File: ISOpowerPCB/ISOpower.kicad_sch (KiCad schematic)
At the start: 12 parts

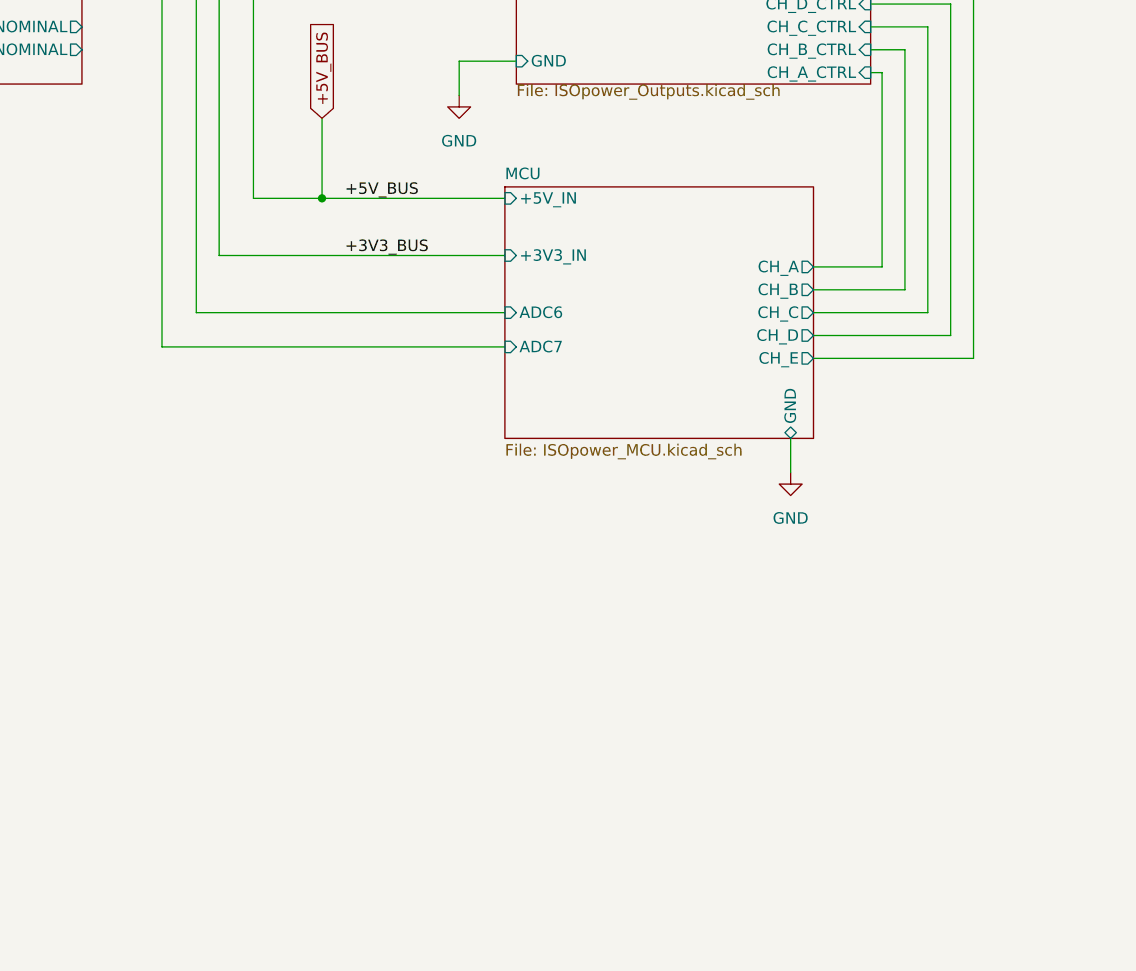
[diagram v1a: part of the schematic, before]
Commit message: modified pcb files
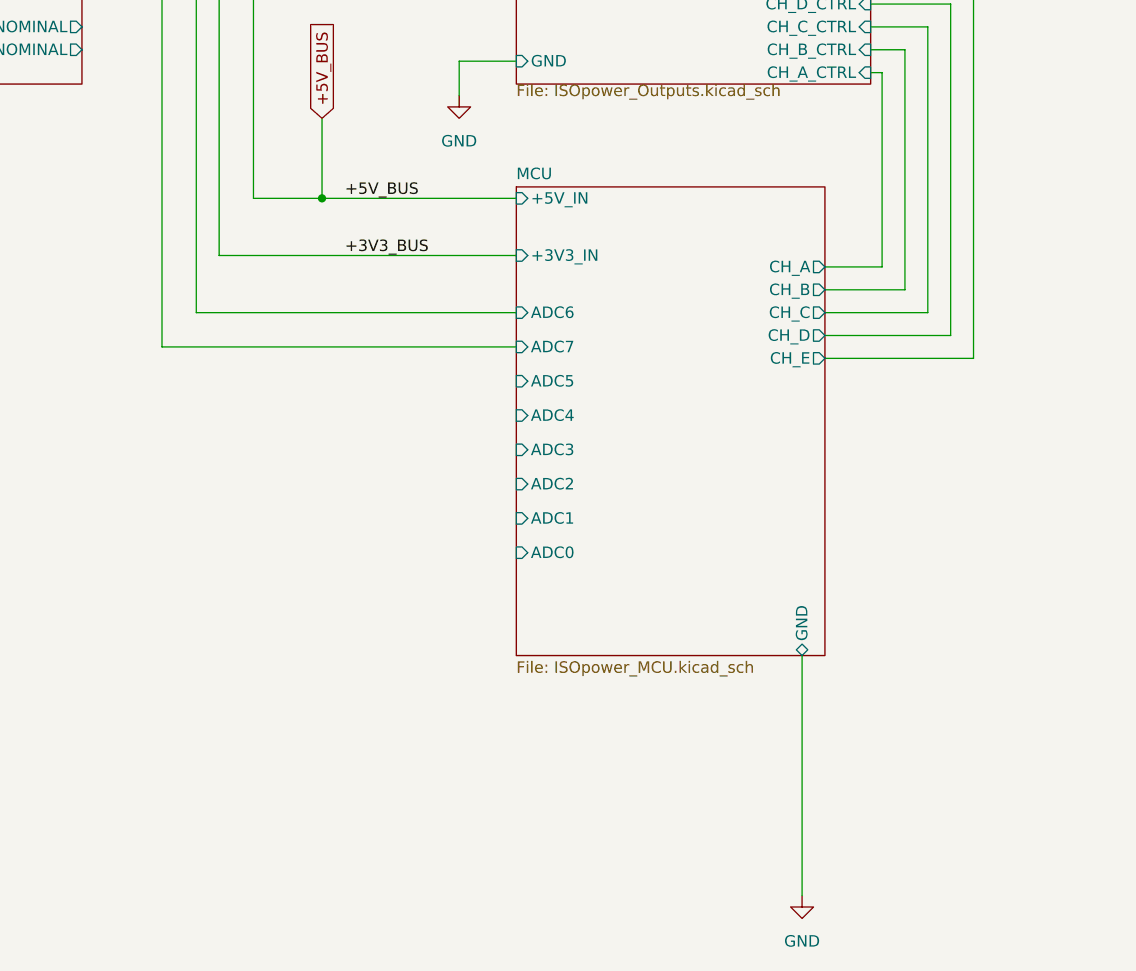
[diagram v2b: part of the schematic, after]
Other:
- sheet MCU ports: added ADC0, ADC1, ADC2, ADC3, ADC4, ADC5; removed none
